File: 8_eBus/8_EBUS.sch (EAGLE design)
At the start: 19 parts, among them IC1 MCP6542, Q1 BC817, X1 AKL18X-02W, X2 ALLSERIALSLAVE

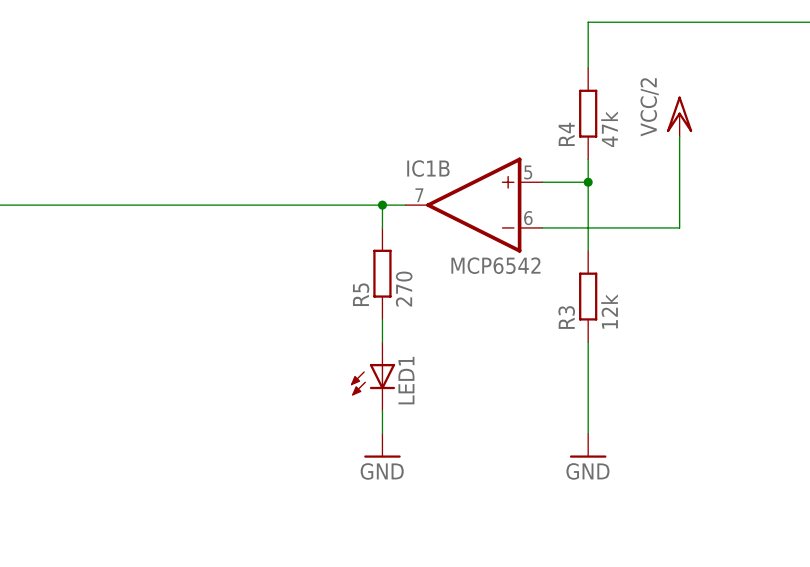
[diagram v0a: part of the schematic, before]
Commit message: Cleanup, front with lib elements
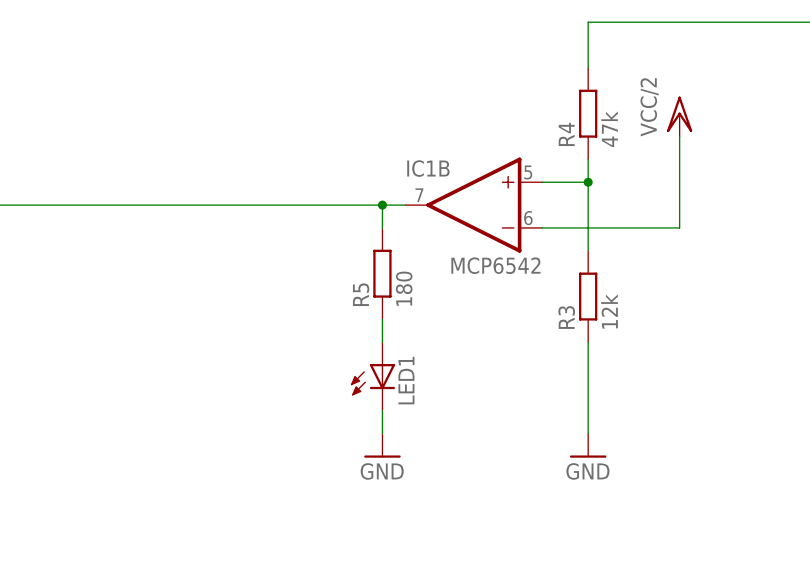
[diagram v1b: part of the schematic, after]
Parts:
- R5: value 270 -> 180
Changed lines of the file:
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@@
 <?xml version="1.0" encoding="utf-8"?>
 <!DOCTYPE eagle SYSTEM "eagle.dtd">
-<eagle version="7.6.0">
+<eagle version="7.7.0">
 <drawing>
 <settings>
@@
 <grid distance="0.1" unitdist="inch" unit="inch" style="lines" multiple="1" display="no" altdistance="0.01" altunitdist="inch" altunit="inch"/>
 <layers>
-<layer number="1" name="Top" color="4" fill="1" visible="no" active="no"/>
-<layer number="2" name="Route2" color="1" fill="3" visible="no" active="no"/>
-<layer number="3" name="Route3" color="4" fill="3" visible="no" active="no"/>
-<layer number="4" name="Route4" color="1" fill="4" visible="no" active="no"/>
-<layer number="5" name="Route5" color="4" fill="4" visible="no" active="no"/>
-<layer number="6" name="Route6" color="1" fill="8" visible="no" active="no"/>
-<layer number="7" name="Route7" color="4" fill="8" visible="no" active="no"/>
-<layer number="8" name="Route8" color="1" fill="2" visible="no" active="no"/>
-<layer number="9" name="Route9" color="4" fill="2" visible="no" active="no"/>
-<layer number="10" name="Route10" color="1" fill="7" visible="no" active="no"/>
-<layer number="11" name="Route11" color="4" fill="7" visible="no" active="no"/>
-<layer number="12" name="Route12" color="1" fill="5" visible="no" active="no"/>
-<layer number="13" name="Route13" color="4" fill="5" visible="no" active="no"/>
-<layer number="14" name="Route14" color="1" fill="6" visible="no" active="no"/>
-<layer number="15" name="Route15" color="4" fill="6" visible="no" active="no"/>
-<layer number="16" name="Bottom" color="1" fill="1" visible="no" active="no"/>
-<layer number="17" name="Pads" color="2" fill="1" visible="no" active="no"/>
-<layer number="18" name="Vias" color="2" fill="1" visible="no" active="no"/>
-<layer number="19" name="Unrouted" color="6" fill="1" visible="no" active="no"/>
-<layer number="20" name="Dimension" color="15" fill="1" visible="no" active="no"/>
-<layer number="21" name="tPlace" color="7" fill="1" visible="no" active="no"/>
-<layer number="22" name="bPlace" color="7" fill="1" visible="no" active="no"/>
-<layer number="23" name="tOrigins" color="15" fill="1" visible="no" active="no"/>
-<layer number="24" name="bOrigins" color="15" fill="1" visible="no" active="no"/>
-<layer number="25" name="tNames" color="7" fill="1" visible="no" active="no"/>
-<layer number="26" name="bNames" color="7" fill="1" visible="no" active="no"/>
-<layer number="27" name="tValues" color="7" fill="1" visible="no" active="no"/>
-<layer number="28" name="bValues" color="7" fill="1" visible="no" active="no"/>
+<layer number="1" name="Top" color="4" fill="1" visible="yes" active="no"/>
+<layer number="2" name="Route2" color="1" fill="3" visible="yes" active="no"/>
+<layer number="3" name="Route3" color="4" fill="3" visible="yes" active="no"/>
+<layer number="4" name="Route4" color="1" fill="4" visible="yes" active="no"/>
+<layer number="5" name="Route5" color="4" fill="4" visible="yes" active="no"/>
+<layer number="6" name="Route6" color="1" fill="8" visible="yes" active="no"/>
+<layer number="7" name="Route7" color="4" fill="8" visible="yes" active="no"/>
+<layer number="8" name="Route8" color="1" fill="2" visible="yes" active="no"/>
+<layer number="9" name="Route9" color="4" fill="2" visible="yes" active="no"/>
+<layer number="10" name="Route10" color="1" fill="7" visible="yes" active="no"/>
+<layer number="11" name="Route11" color="4" fill="7" visible="yes" active="no"/>
+<layer number="12" name="Route12" color="1" fill="5" visible="yes" active="no"/>
+<layer number="13" name="Route13" color="4" fill="5" visible="yes" active="no"/>
+<layer number="14" name="Route14" color="1" fill="6" visible="yes" active="no"/>
+<layer number="15" name="Route15" color="4" fill="6" visible="yes" active="no"/>
+<layer number="16" name="Bottom" color="1" fill="1" visible="yes" active="no"/>
+<layer number="17" name="Pads" color="2" fill="1" visible="yes" active="no"/>
+<layer number="18" name="Vias" color="2" fill="1" visible="yes" active="no"/>
+<layer number="19" name="Unrouted" color="6" fill="1" visible="yes" active="no"/>
+<layer number="20" name="Dimension" color="15" fill="1" visible="yes" active="no"/>
+<layer number="21" name="tPlace" color="7" fill="1" visible="yes" active="no"/>
+<layer number="22" name="bPlace" color="7" fill="1" visible="yes" active="no"/>
+<layer number="23" name="tOrigins" color="15" fill="1" visible="yes" active="no"/>
+<layer number="24" name="bOrigins" color="15" fill="1" visible="yes" active="no"/>
+<layer number="25" name="tNames" color="7" fill="1" visible="yes" active="no"/>
+<layer number="26" name="bNames" color="7" fill="1" visible="yes" active="no"/>
+<layer number="27" name="tValues" color="7" fill="1" visible="yes" active="no"/>
+<layer number="28" name="bValues" color="7" fill="1" visible="yes" active="no"/>
 <layer number="29" name="tStop" color="7" fill="3" visible="no" active="no"/>
 <layer number="30" name="bStop" color="7" fill="6" visible="no" active="no"/>
@@
 <layer number="35" name="tGlue" color="7" fill="4" visible="no" active="no"/>
 <layer number="36" name="bGlue" color="7" fill="5" visible="no" active="no"/>
-<layer number="37" name="tTest" color="7" fill="1" visible="no" active="no"/>
-<layer number="38" name="bTest" color="7" fill="1" visible="no" active="no"/>
+<layer number="37" name="tTest" color="7" fill="1" visible="yes" active="no"/>
+<layer number="38" name="bTest" color="7" fill="1" visible="yes" active="no"/>
 <layer number="39" name="tKeepout" color="4" fill="11" visible="no" active="no"/>
 <layer number="40" name="bKeepout" color="1" fill="11" visible="no" active="no"/>
@@
 <layer number="44" name="Drills" color="7" fill="1" visible="no" active="no"/>
 <layer number="45" name="Holes" color="7" fill="1" visible="no" active="no"/>
-<layer number="46" name="Milling" color="3" fill="1" visible="no" active="no"/>
-<layer number="47" name="Measures" color="7" fill="1" visible="no" active="no"/>
-<layer number="48" name="Document" color="7" fill="1" visible="no" active="no"/>
-<layer number="49" name="Reference" color="7" fill="1" visible="no" active="no"/>
-<layer number="50" name="dxf" color="7" fill="1" visible="no" active="no"/>
-<layer number="51" name="tDocu" color="7" fill="1" visible="no" active="no"/>
-<layer number="52" name="bDocu" color="7" fill="1" visible="no" active="no"/>
-<layer number="53" name="tGND_GNDA" color="7" fill="9" visible="no" active="no"/>
-<layer number="54" name="bGND_GNDA" color="1" fill="9" visible="no" active="no"/>
-<layer number="56" name="wert" color="7" fill="1" visible="no" active="no"/>
-<layer number="57" name="tCAD" color="7" fill="1" visible="no" active="no"/>
-<layer number="58" name="bCAD" color="11" fill="1" visible="no" active="no"/>
-<layer number="59" name="tCarbon" color="7" fill="1" visible="no" active="no"/>
-<layer number="60" name="bCarbon" color="7" fill="1" visible="no" active="no"/>
-<layer number="61" name="pt_docu" color="7" fill="0" visible="no" active="no"/>
+<layer number="46" name="Milling" color="3" fill="1" visible="yes" active="no"/>
+<layer number="47" name="Measures" color="7" fill="1" visible="yes" active="no"/>
+<layer number="48" name="Document" color="7" fill="1" visible="yes" active="no"/>
+<layer number="49" name="Reference" color="7" fill="1" visible="yes" active="no"/>
+<layer number="50" name="dxf" color="7" fill="1" visible="yes" active="no"/>
+<layer number="51" name="tDocu" color="7" fill="1" visible="yes" active="no"/>
+<layer number="52" name="bDocu" color="7" fill="1" visible="yes" active="no"/>
+<layer number="53" name="tGND_GNDA" color="7" fill="9" visible="yes" active="no"/>
+<layer number="54" name="bGND_GNDA" color="1" fill="9" visible="yes" active="no"/>
+<layer number="56" name="wert" color="7" fill="1" visible="yes" active="no"/>
+<layer number="57" name="tCAD" color="7" fill="1" visible="yes" active="no"/>
+<layer number="58" name="bCAD" color="11" fill="1" visible="yes" active="no"/>
+<layer number="59" name="tCarbon" color="7" fill="1" visible="yes" active="no"/>
+<layer number="60" name="bCarbon" color="7" fill="1" visible="yes" active="no"/>
+<layer number="61" name="pt_docu" color="7" fill="0" visible="yes" active="no"/>
 <layer number="90" name="Modules" color="5" fill="1" visible="yes" active="yes"/>
 <layer number="91" name="Nets" color="2" fill="1" visible="yes" active="yes"/>
@@
 <part name="LED1" library="led" deviceset="LED" device="CHIPLED_0805"/>
 <part name="GND8" library="supply1" deviceset="GND" device=""/>
-<part name="R5" library="rcl" deviceset="R-EU_" device="R0805" value="270"/>
+<part name="R5" library="rcl" deviceset="R-EU_" device="R0805" value="180"/>
 <part name="GND9" library="supply1" deviceset="GND" device=""/>
 <part name="P+6" library="supply1" deviceset="VCC/2" device=""/>
